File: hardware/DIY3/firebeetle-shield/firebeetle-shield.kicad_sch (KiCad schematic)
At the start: 6 parts, among them J1 Conn_01x14_Female, J2 Conn_01x06_Female (DS3231), J3 Conn_01x06_Female (microSD), J4 Conn_01x04_Male (JST to MS580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, J5 Conn_01x18_Female

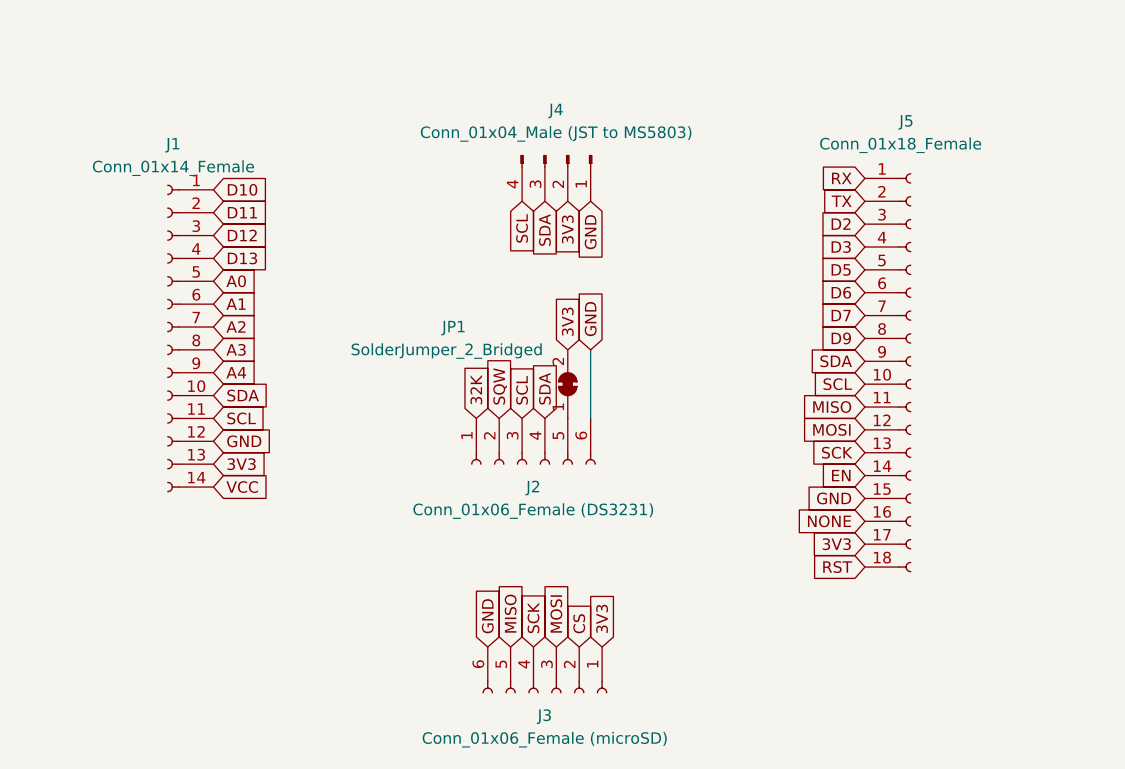
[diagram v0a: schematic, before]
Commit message: Finish shield design
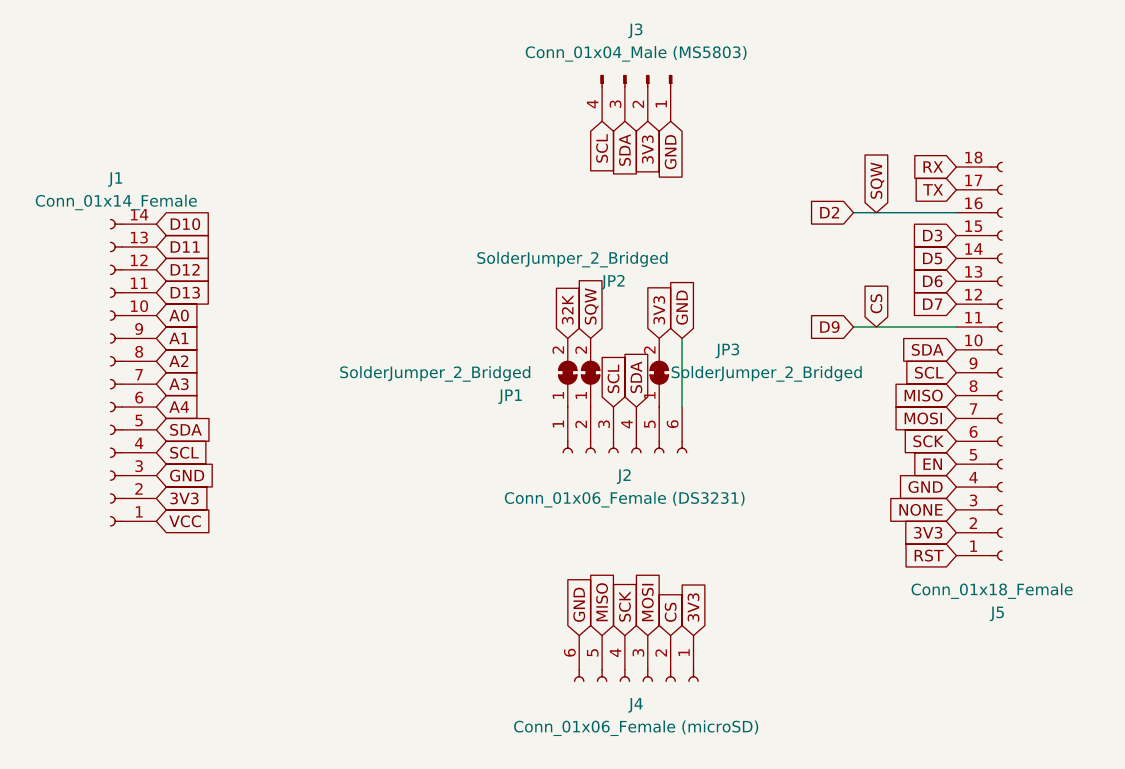
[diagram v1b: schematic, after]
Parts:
- added JP1, JP2: SolderJumper_2_Bridged, Jumper:SolderJumper-2_P1.3mm_Bridged_RoundedPad1.0x1.5mm, symbol Jumper:SolderJumper_2_Bridged
- J3: renamed from J4; value Conn_01x04_Male (JST to MS5803) -> Conn_01x04_Male (MS5803)
- renumbered J3 to J4, JP1 to JP3
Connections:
- net D9 is gone; now on net MISO: J5.8 (Pin_8)
- net 32K: now also JP1.2 (B); no longer J2.1 (Pin_1)
- net 3V3: now also J1.2 (Pin_2), J5.2 (Pin_2); no longer J1.13 (Pin_13), J5.17 (Pin_17)
- net A0: now also J1.10 (Pin_10); no longer J1.5 (Pin_5)
- net A1: now also J1.9 (Pin_9); no longer J1.6 (Pin_6)
- net A2: now also J1.8 (Pin_8); no longer J1.7 (Pin_7)
- net A3: now also J1.7 (Pin_7); no longer J1.8 (Pin_8)
- net A4: now also J1.6 (Pin_6); no longer J1.9 (Pin_9)
- net CS: now also J5.11 (Pin_11)
- net D10: now also J1.14 (Pin_14); no longer J1.1 (Pin_1)
- net D11: now also J1.13 (Pin_13); no longer J1.2 (Pin_2)
- net D12: now also J1.12 (Pin_12); no longer J1.3 (Pin_3)
- net D13: now also J1.11 (Pin_11); no longer J1.4 (Pin_4)
- net D2: now also J5.16 (Pin_16), JP2.2 (B); no longer J5.3 (Pin_3)
- net D3: now also J5.15 (Pin_15); no longer J5.4 (Pin_4)
- net D5: now also J5.14 (Pin_14); no longer J5.5 (Pin_5)
- net D6: now also J5.13 (Pin_13); no longer J5.6 (Pin_6)
- net D7: now also J5.12 (Pin_12); no longer J5.7 (Pin_7)
- net EN: now also J5.5 (Pin_5); no longer J5.14 (Pin_14)
- net GND: now also J1.3 (Pin_3), J5.4 (Pin_4); no longer J1.12 (Pin_12), J5.15 (Pin_15)
- net MISO: no longer J5.11 (Pin_11)
- net MOSI: now also J5.7 (Pin_7); no longer J5.12 (Pin_12)
- net NONE: now also J5.3 (Pin_3); no longer J5.16 (Pin_16)
- net RST: now also J5.1 (Pin_1); no longer J5.18 (Pin_18)
- net RX: now also J5.18 (Pin_18); no longer J5.1 (Pin_1)
- net SCK: now also J5.6 (Pin_6); no longer J5.13 (Pin_13)
- net SCL: now also J1.4 (Pin_4), J5.9 (Pin_9); no longer J1.11 (Pin_11), J5.10 (Pin_10)
- net SDA: now also J1.5 (Pin_5), J5.10 (Pin_10); no longer J1.10 (Pin_10), J5.9 (Pin_9)
- net TX: now also J5.17 (Pin_17); no longer J5.2 (Pin_2)
- net VCC: now also J1.1 (Pin_1); no longer J1.14 (Pin_14)
- net SQW: no longer names the net of J2.2 (Pin_2)
- net SQW: now also JP2.1 (A)
- new net: J2.1 (Pin_1), JP1.1 (A)
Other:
- moved on the sheet: J1, J2, J3, J4, J5, JP3
